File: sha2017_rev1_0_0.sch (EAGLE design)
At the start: 202 parts, among them IC1 CP210X_USB_UART, IC2 AP7215, IC3 ESP32WROOM32, IC4 TP4056, IC5 AMS1117, M1 MOTOR10MM, Q1 MMBT2222A, Q2 MMBT2222A, Q3 MMBT2222A, Q4 MMBT2222A, Q5 SI1304 BDL, Q6 MMBT2222A, T1 MOSFET-PCHANNEL, T2 MOSFET-PCHANNEL, T3 MOSFET-PCHANNEL, U1 MPR121QR2, X2 2908-05WB-MG, X4 JST-PH3

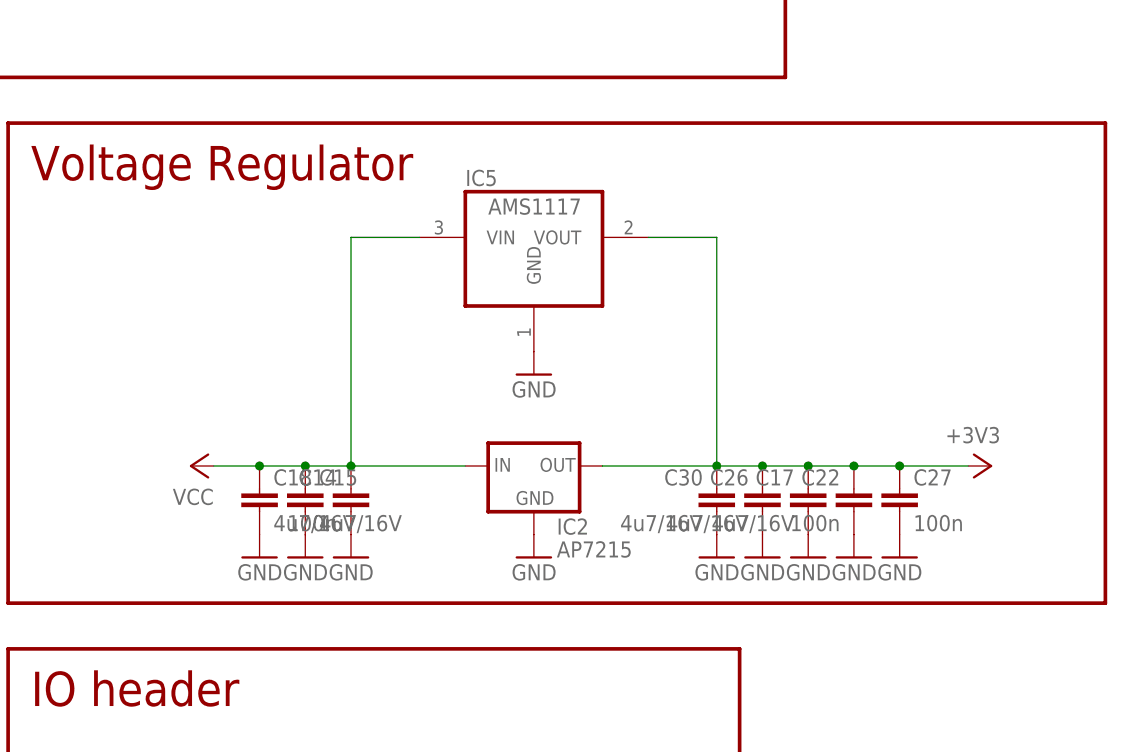
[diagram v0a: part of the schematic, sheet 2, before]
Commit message: Replace vreg
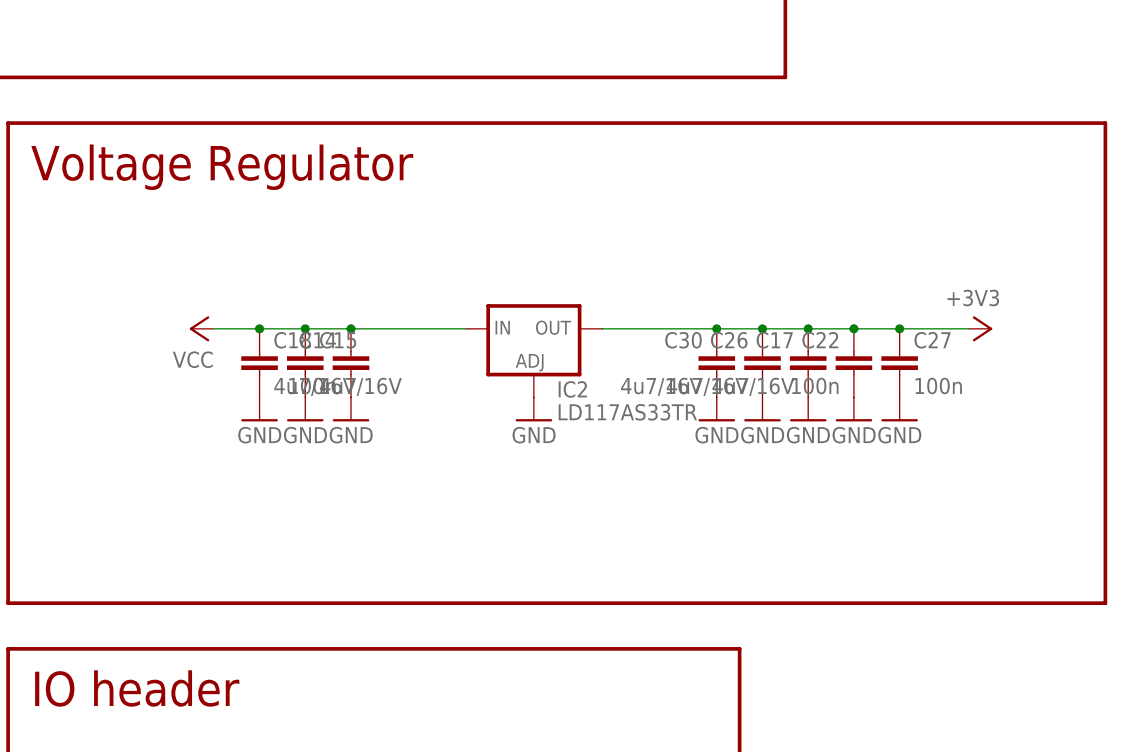
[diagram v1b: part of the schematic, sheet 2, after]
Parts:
- removed IC5: AMS1117, burr-brown:REG1117
- IC2: value AP7215 -> LD117AS33TR; device badge:AP7215 -> v-reg:LD117AS33TR
- R2: device resistor:R-EU_R1206 -> rcl:R-EU_R1206
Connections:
- net +3V3: no longer IC5.VOUT
- net GND: now also IC2.ADJ; no longer IC2.GND, IC5.GND
- net VCC: no longer IC5.VIN
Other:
- moved on the sheet: C14, C15, C17, C18, C22, C26, C27, C30, IC2
